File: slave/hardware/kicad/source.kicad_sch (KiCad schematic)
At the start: 47 parts, among them IC1 L6982C50, IC2 L6982C33, IC3 STEF12SGR, IC4 STEF12SGR, Q1 IPD50P04P4L-11

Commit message: feat(HW): add footprints and configure component properties
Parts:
- IC1, IC2: footprint SOIC127P600X175-8N -> Datalogger:SOIC127P600X175-8N
- IC3, IC4: footprint SOP65P280X100-8N -> Datalogger:SOIC127P600X175-8N
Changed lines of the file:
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@@
 			)
 		)
-		(property "Footprint" "SOP65P280X100-8N"
+		(property "Footprint" "Datalogger:SOIC127P600X175-8N"
 			(at 220.98 149.53 0)
 			(hide yes)
@@
 			)
 		)
-		(property "Footprint" "SOIC127P600X175-8N"
+		(property "Footprint" "Datalogger:SOIC127P600X175-8N"
 			(at 152.4 146.99 0)
 			(hide yes)
@@
 			)
 		)
-		(property "Footprint" "SOIC127P600X175-8N"
+		(property "Footprint" "Datalogger:SOIC127P600X175-8N"
 			(at 152.4 188.9 0)
 			(hide yes)
@@
 			)
 		)
-		(property "Footprint" "SOP65P280X100-8N"
+		(property "Footprint" "Datalogger:SOIC127P600X175-8N"
 			(at 220.98 191.44 0)
 			(hide yes)

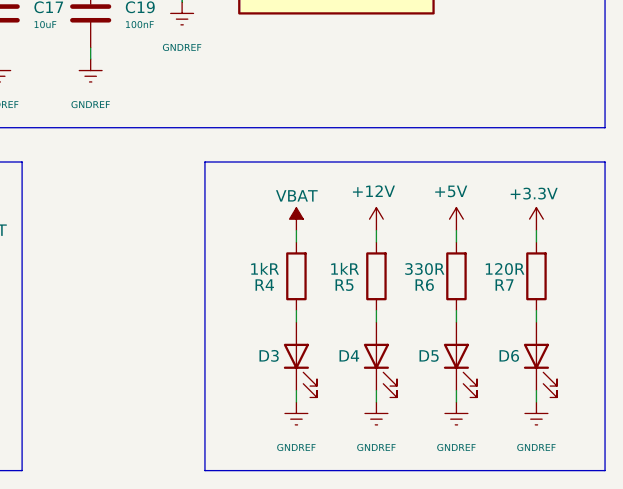
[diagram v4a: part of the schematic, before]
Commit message: feat(HW): finalize schematic design
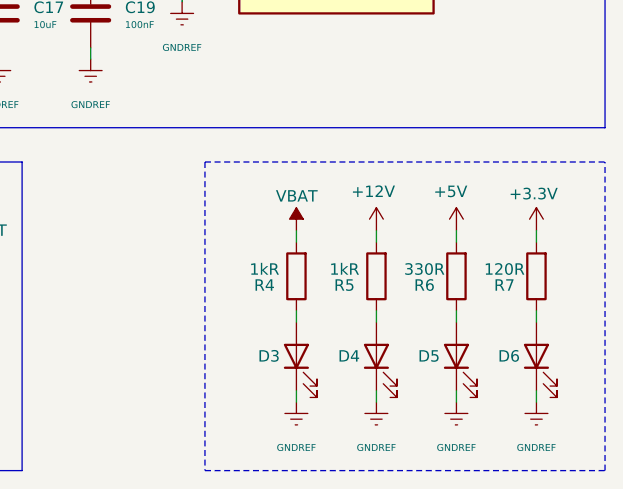
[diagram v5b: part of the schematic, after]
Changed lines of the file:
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@@
 		(stroke
 			(width 0)
-			(type default)
+			(type dash_dot_dot)
 		)
 	)
@@
 		(stroke
 			(width 0)
-			(type default)
+			(type dash_dot_dot)
 		)
 	)
@@
 		(stroke
 			(width 0)
-			(type default)
+			(type dash_dot_dot)
 		)
 	)
@@
 		(stroke
 			(width 0)
-			(type default)
-		)
-	)
+			(type dash_dot_dot)
+		)
+	)
